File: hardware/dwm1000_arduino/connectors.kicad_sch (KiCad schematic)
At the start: 10 parts, among them J1 Barrel_Jack, J2 PWR_IN, J3 UART, J4 SPI, J5 NEO_OUT, J6 Conn_01x06_Male

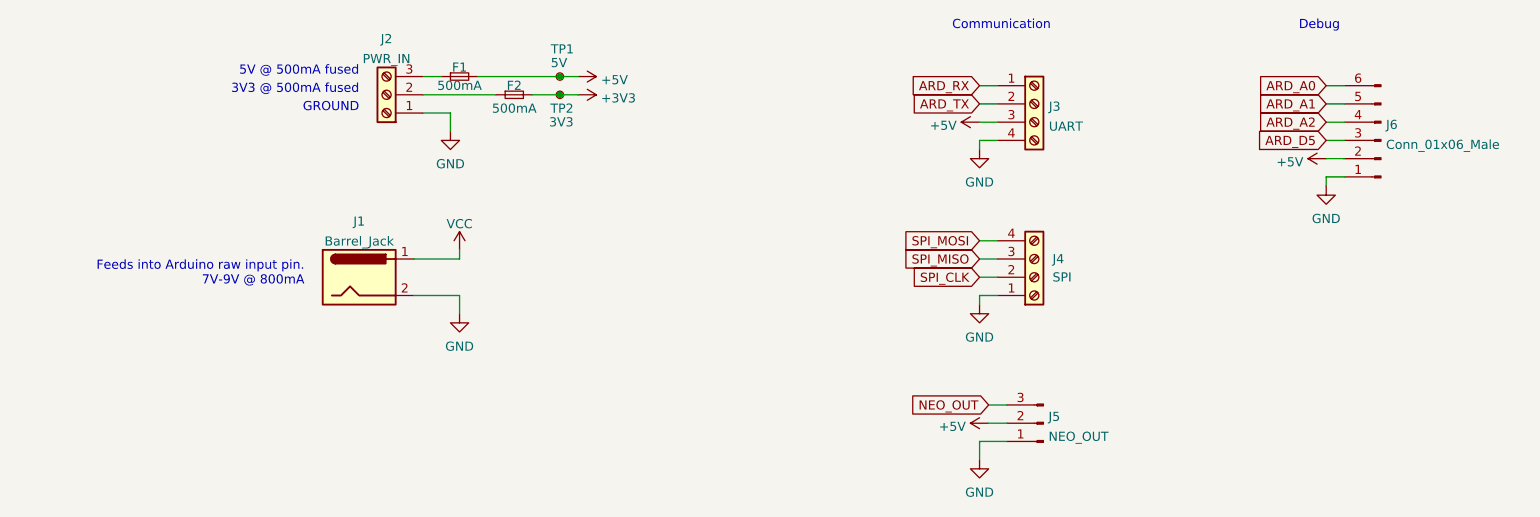
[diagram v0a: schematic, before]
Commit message: finixh schematic and first pass layout
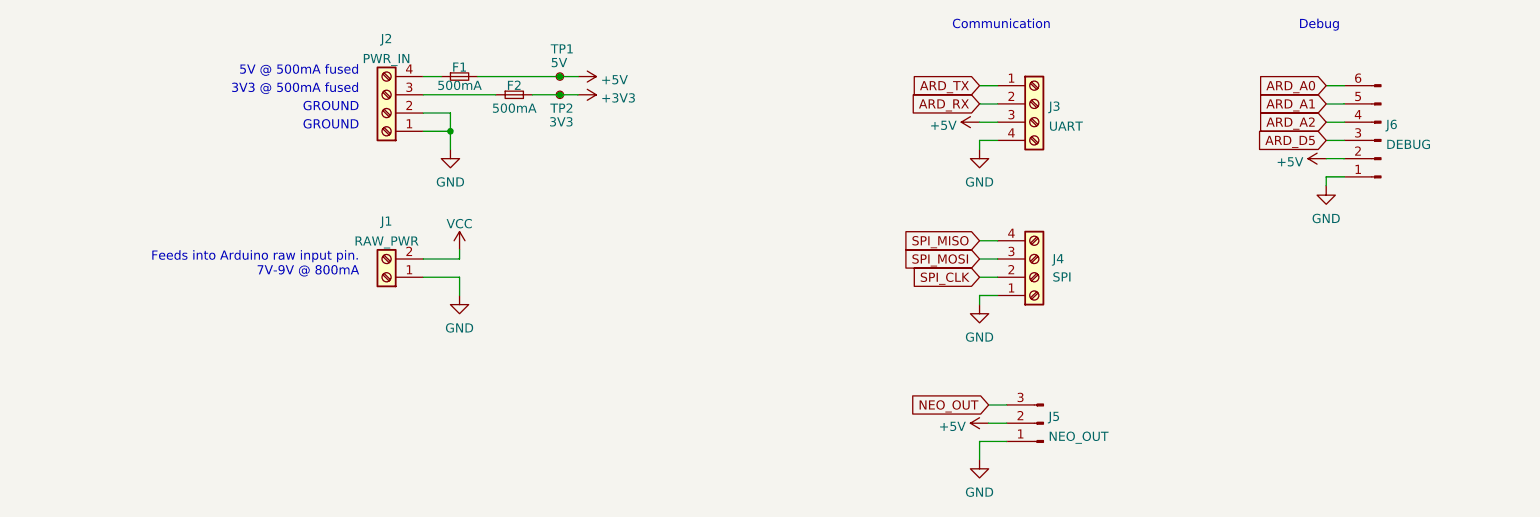
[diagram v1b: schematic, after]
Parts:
- removed J1: Barrel_Jack, symbol Connector:Barrel_Jack
- removed J2: PWR_IN, symbol Connector:Screw_Terminal_01x03
- added J1: RAW_PWR, TerminalBlock_Phoenix:TerminalBlock_Phoenix_PT-1,5-2-3.5-H_1x02_P3.50mm_Horizontal, symbol Connector:Screw_Terminal_01x02
- added J2: PWR_IN, TerminalBlock_Phoenix:TerminalBlock_Phoenix_PT-1,5-4-3.5-H_1x04_P3.50mm_Horizontal, symbol Connector:Screw_Terminal_01x04
- F1, F2: footprint (none) -> Fuse:Fuse_1206_3216Metric_Pad1.42x1.75mm_HandSolder; DigiKey (none) -> 507-1802-6-ND
- J3, J4: footprint (none) -> TerminalBlock_Phoenix:TerminalBlock_Phoenix_PT-1,5-4-3.5-H_1x04_P3.50mm_Horizontal; DigiKey (none) -> 277-1860-ND
- J5: footprint (none) -> Connector_PinHeader_2.54mm:PinHeader_1x03_P2.54mm_Vertical
- J6: value Conn_01x06_Male -> DEBUG; footprint (none) -> Connector_PinHeader_2.54mm:PinHeader_1x06_P2.54mm_Vertical
- TP1, TP2: footprint (none) -> TestPoint:TestPoint_Pad_D2.5mm
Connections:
- net ARD_RX: now also J3.2 (Pin_2); no longer J3.1 (Pin_1)
- net ARD_TX: now also J3.1 (Pin_1); no longer J3.2 (Pin_2)
- net GND: now also J1.1 (Pin_1), J2.1 (Pin_1), J2.2 (Pin_2)
- net SPI_MISO: now also J4.4 (Pin_4); no longer J4.3 (Pin_3)
- net SPI_MOSI: now also J4.3 (Pin_3); no longer J4.4 (Pin_4)
- net VCC: now also J1.2 (Pin_2)
- net at F2.1: now also J2.3 (Pin_3)
- net at F1.1: now also J2.4 (Pin_4)
